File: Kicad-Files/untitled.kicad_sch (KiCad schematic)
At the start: 13 parts, among them U3 TPS74401

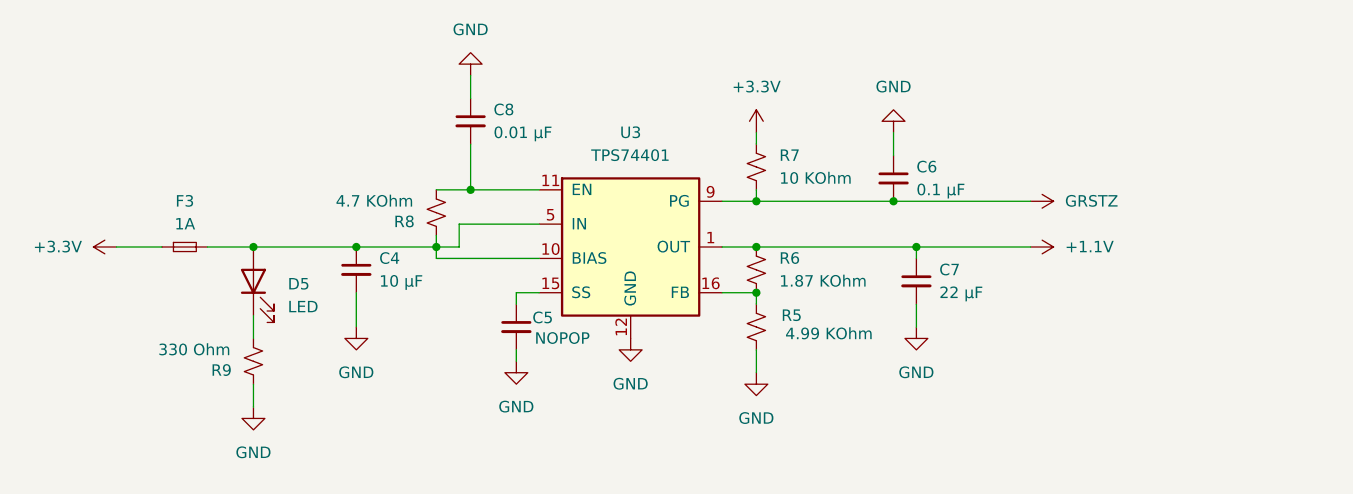
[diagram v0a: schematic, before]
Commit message: Updated schematics for 1.1V circuit
Signed-off-by: Jakub Sobota <jakub.sobota@3mdeb.com>
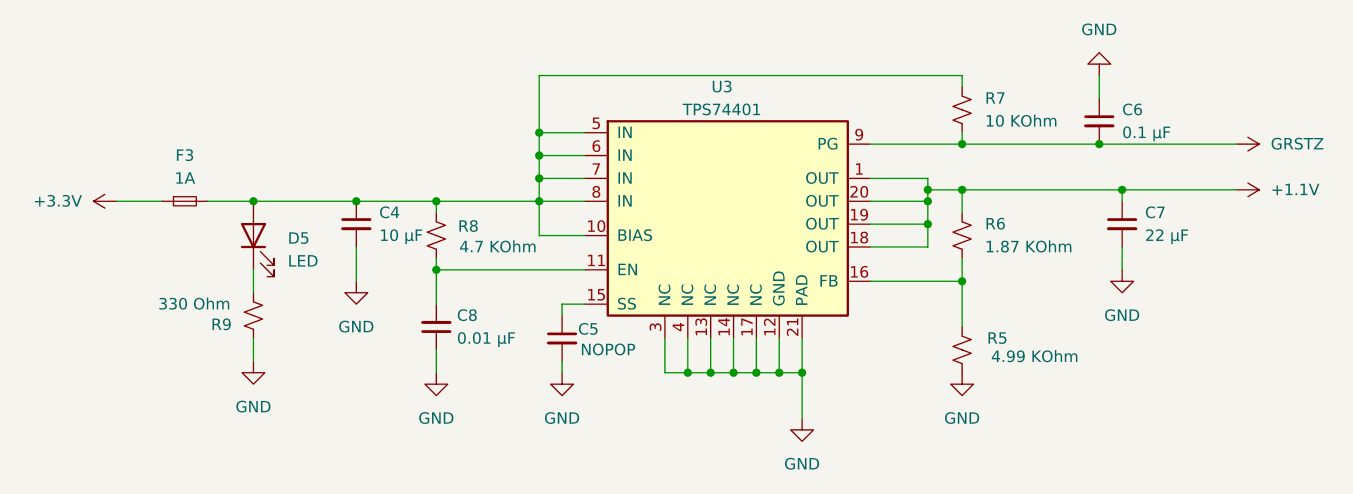
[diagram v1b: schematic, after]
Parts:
- D5: footprint Diode_SMD:D_0603_1608Metric_Pad1.05x0.95mm_HandSolder -> LED_SMD:LED_0603_1608Metric_Pad1.05x0.95mm_HandSolder
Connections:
- net +1.1V: now also U3.18 (OUT), U3.19 (OUT), U3.20 (OUT)
- net +3.3V: no longer R7.1
- net GND: now also U3.13 (NC), U3.14 (NC), U3.17 (NC), U3.21 (PAD), U3.3 (NC), U3.4 (NC)
- net at C4.1, D5.2 (A), F3.2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: now also R7.1, U3.6 (IN), U3.7 (IN), U3.8 (IN)
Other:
- moved on the sheet: C4, C5, C6, C7, C8, D5, F3, R5, R6, R7, R8, R9
